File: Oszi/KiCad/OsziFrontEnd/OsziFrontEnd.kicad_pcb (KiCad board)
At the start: 2 copper layers, 150.4 x 65.4 mm, 29 parts, among them J1 Conn_Coaxial, J2 Conn_Coaxial, J3 Conn_01x03_Pin, J4 Conn_01x03_Pin, J5 USB_C_Receptacle_PowerOnly_6P, U1 MCP6002-xP, U2 MCP6002-xP, U3 NUCLEO-L432KC

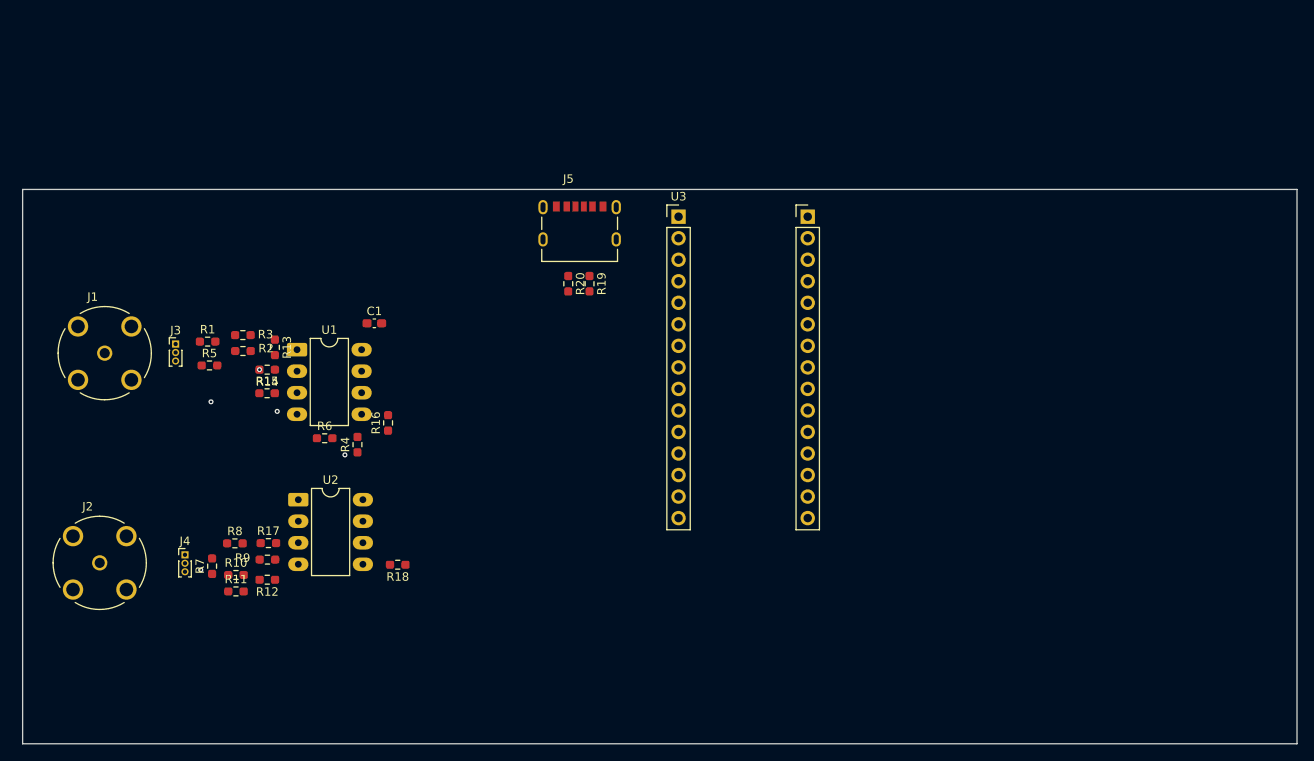
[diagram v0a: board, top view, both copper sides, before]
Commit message: finished layout
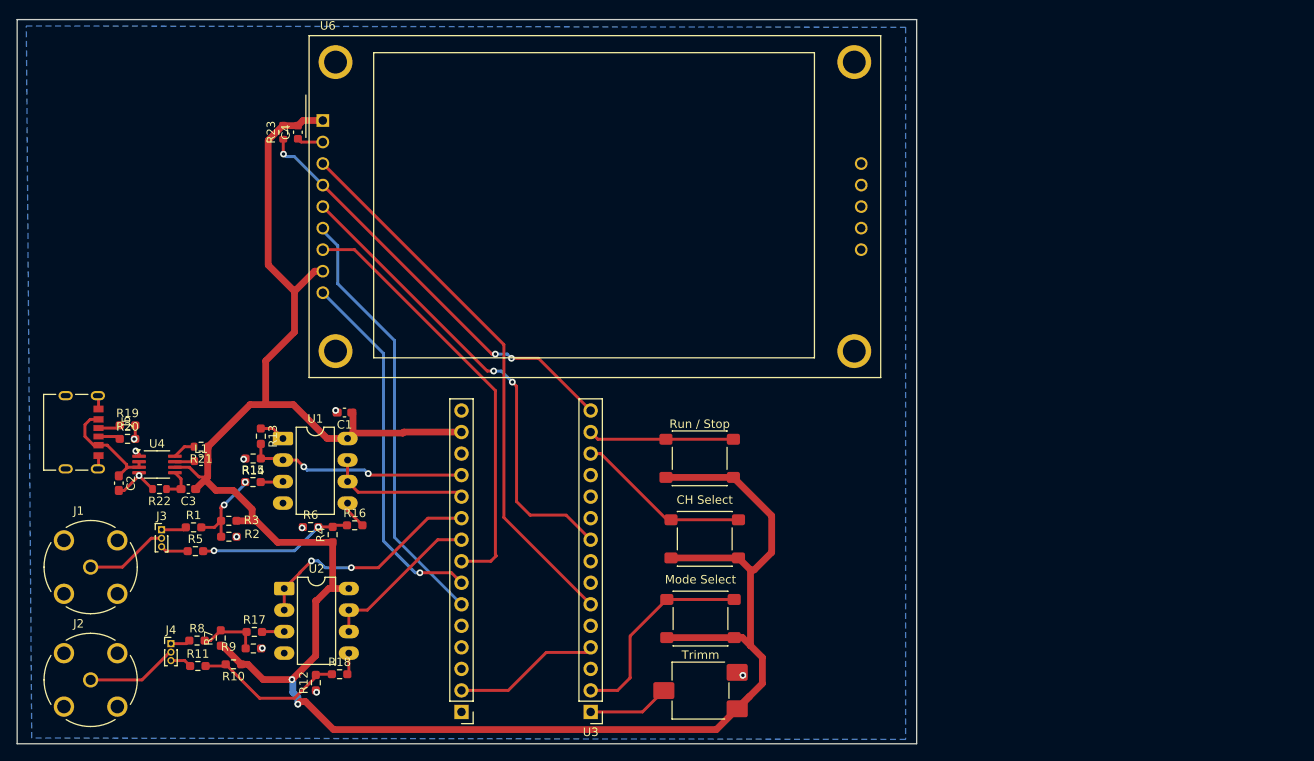
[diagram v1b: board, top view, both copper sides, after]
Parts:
- added C2: 10u, Capacitor_SMD:C_0603_1608Metric_Pad1.08x0.95mm_HandSolder, F.Cu at (88.3, 70.7)
- added C3: 22u, Capacitor_SMD:C_0603_1608Metric_Pad1.08x0.95mm_HandSolder, F.Cu at (96.5, 71.4)
- added C4: 12p, Capacitor_SMD:C_0603_1608Metric, F.Cu at (109.4, 29.3)
- added CH Select: SW_Push, Button_Switch_SMD:SW_SPST_PTS645Sx43SMTR92, F.Cu at (157.4, 77.3)
- added L1: 2.2u, Inductor_SMD:L_0603_1608Metric, F.Cu at (98.0, 68.1)
- added Mode Select: SW_Push, Button_Switch_SMD:SW_SPST_PTS645Sx43SMTR92, F.Cu at (156.9, 86.7)
- added R21: 330k, Resistor_SMD:R_0603_1608Metric, F.Cu at (98.0, 66.4)
- added R22: 100k, Resistor_SMD:R_0603_1608Metric, F.Cu at (93.1, 71.4)
- added R23: 10k, Resistor_SMD:R_0603_1608Metric, F.Cu at (107.7, 29.3)
- added Run / Stop: SW_Push, Button_Switch_SMD:SW_SPST_PTS645Sx43SMTR92, F.Cu at (156.8, 67.8)
- added Trimm: R_Potentiometer, Potentiometer_SMD:Potentiometer_ACP_CA6-VSMD_Vertical, F.Cu at (156.9, 95.2)
- added U4: TPS62160DGK, Package_SO:MSOP-8_3x3mm_P0.65mm, F.Cu at (92.8, 68.5)
- added U6: CR2013-MI2120, Display:CR2013-MI2120, F.Cu at (112.3, 27.9)
- moved J5 64.8 mm to (82.0, 64.7), turned to -90 degrees
- moved U3 59.3 mm to (143.9, 97.7), turned to 180 degrees
- moved R19 57.0 mm to (89.3, 63.9), turned to 0 degrees
- moved R20 55.1 mm to (89.3, 65.5), turned to 0 degrees
- moved J1 25.3 mm to (85.0, 80.6)
- moved R3 22.0 mm to (101.2, 75.2)
- moved J3 22.0 mm to (93.3, 76.2)
- moved R1 22.0 mm to (97.1, 75.9)
- moved R2 22.0 mm to (101.3, 77.0)
- moved R5 22.0 mm to (97.3, 78.8)
- moved R18 14.6 mm to (114.3, 93.3), turned to 0 degrees
- moved J2 13.9 mm to (85.0, 93.9)
- moved R12 13.4 mm to (111.5, 94.3), turned to 90 degrees
- moved R16 12.7 mm to (116.1, 75.7), turned to 0 degrees
- moved R8 12.3 mm to (97.5, 89.3)
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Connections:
- net /AnalogesFrontEnd/3V3 renamed 3V3
- J5 pad A9: USB-COutZu5V -> /powerSupplie/USB-cOut
- J5 pad B9: USB-COutZu5V -> /powerSupplie/USB-cOut
- R1 pad 1: /AnalogesFrontEnd/Vin-10;10CH1 -> /AnalogesFrontEnd/Vin-1;1CH1
- U3 pad CN3_1: unconnected-(U3A-PA9-PadCN3_1) -> Net-(U3A-PA9)
- U3 pad CN3_12: unconnected-(U3A-PA8-PadCN3_12) -> /muC/EINT
- U3 pad CN3_13: unconnected-(U3A-PA11-PadCN3_13) -> Net-(U3A-PA11)
- U3 pad CN3_14: unconnected-(U3A-PB5-PadCN3_14) -> Net-(U3A-PB5)
- U3 pad CN3_15: unconnected-(U3A-PB4-PadCN3_15) -> /Display/DRs
- U3 pad CN3_2: unconnected-(U3A-PA10-PadCN3_2) -> Net-(U3A-PA10)
- U3 pad CN3_6: /AnalogesFrontEnd/ADC_CH1_1V -> /Display/DCS
- U3 pad CN3_7: unconnected-(U3A-PB7-PadCN3_7) -> /muC/ERs
- U3 pad CN3_8: unconnected-(U3A-PB6-PadCN3_8) -> /muC/ECS
- U3 pad CN3_9: /AnalogesFrontEnd/ADC_CH1_10V -> /Display/DD/C
- U3 pad CN4_10: unconnected-(U3B-PA3-PadCN4_10) -> /AnalogesFrontEnd/ADC_CH2_36V
- U3 pad CN4_11: /AnalogesFrontEnd/ADC_CH2_10V -> /AnalogesFrontEnd/ADC_CH1_10V
- U3 pad CN4_12: /AnalogesFrontEnd/ADC_CH2_36V -> /AnalogesFrontEnd/ADC_CH1_1V
- U3 pad CN4_4: USB-COutZu5V -> unconnected-(U3B-+5V-PadCN4_4)
- U3 pad CN4_6: unconnected-(U3B-PA7-PadCN4_6) -> /Display/DMOSI
- U3 pad CN4_7: unconnected-(U3B-PA6-PadCN4_7) -> /Display/DMISO
- U3 pad CN4_8: unconnected-(U3B-PA5-PadCN4_8) -> /Display/DSCK
- U3 pad CN4_9: unconnected-(U3B-PA4-PadCN4_9) -> /AnalogesFrontEnd/ADC_CH2_10V
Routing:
- net 3V3: track 0.00 -> 263.5 mm
- net /Display/DCS: track 0.00 -> 65.1 mm
- net /Display/DD/C: track 0.00 -> 55.8 mm, vias 0 -> 2
- net /Display/DMOSI: track 0.00 -> 51.2 mm
- net /Display/DSCK: track 0.00 -> 51.1 mm
- net /Display/DRs: track 0.00 -> 50.5 mm, vias 0 -> 3
- net /Display/DMISO: track 0.00 -> 43.5 mm, vias 0 -> 1
- net /AnalogesFrontEnd/ADC_CH2_36V: track 0.00 -> 27.8 mm, vias 0 -> 2
- net /AnalogesFrontEnd/ADC_CH1_1V: track 0.00 -> 26.2 mm, vias 0 -> 2
- net Net-(U3A-PA10): track 0.00 -> 24.3 mm
- net Net-(U3A-PA11): track 0.00 -> 20.7 mm
- net /AnalogesFrontEnd/ADC_CH2_10V: track 0.00 -> 19.3 mm
- net /AnalogesFrontEnd/Vout-10;10CH1: track 0.00 -> 18.5 mm, vias 0 -> 2
- net /AnalogesFrontEnd/Vout-10;10CH2: track 0.00 -> 17.9 mm
- net GNDD: track 0.00 -> 17.3 mm
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- added copper zone on B.Cu, net GND
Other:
- board size 150.4 x 65.4 mm -> 106.1 x 85.4 mm
